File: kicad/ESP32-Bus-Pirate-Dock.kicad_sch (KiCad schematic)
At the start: 23 parts, among them CN1 HX25418-10WA, J1 Conn_01x10V, J2 Conn_01x22, J3 Conn_01x22, J5 Conn_01x22, J6 Conn_01x22, U1 ESP32-S3-DEVKITC-1-N8R2, U2 AMS1117-1.8, U3 FXMA108

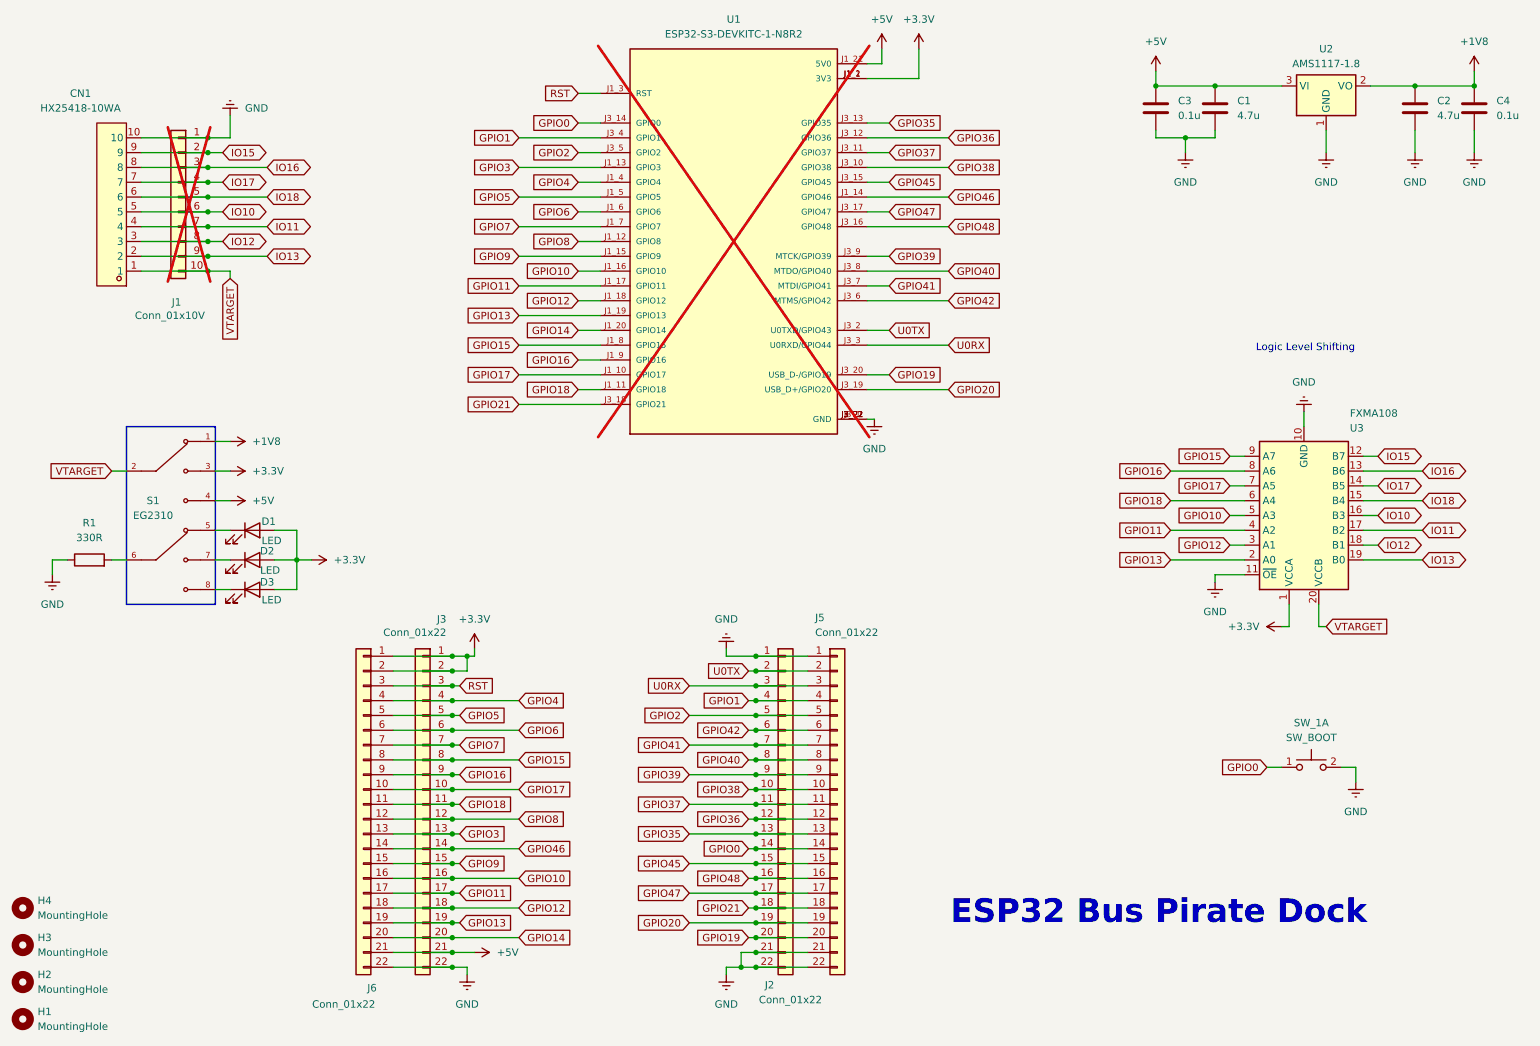
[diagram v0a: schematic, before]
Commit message: PCB reassignment
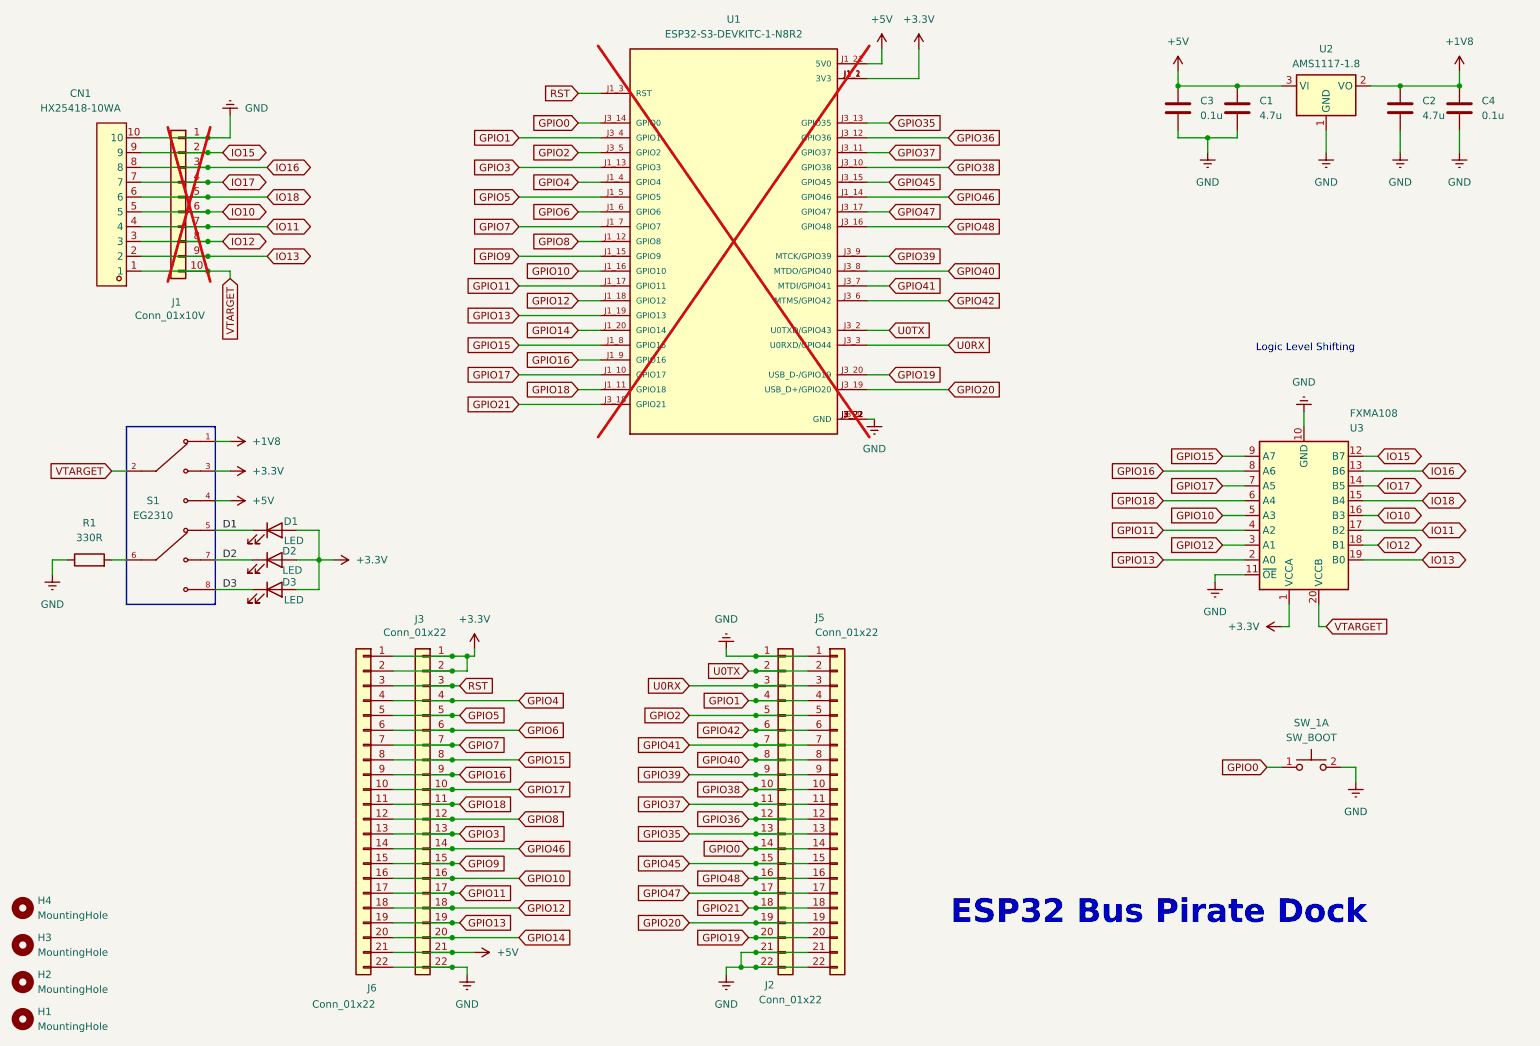
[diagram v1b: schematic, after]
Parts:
- H1, H2, H3, H4: footprint MountingHole:MountingHole_3.2mm_M3 -> MountingHole:MountingHole_3.2mm_M3_DIN965_Pad_TopBottom
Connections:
- net D3: now reaches D3.1 (K), S1.8
- net D1: now reaches D1.1 (K), S1.5
- net D2: now reaches D2.1 (K), S1.7
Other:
- moved on the sheet: C1, C2, C3, C4, D1, D2, D3
